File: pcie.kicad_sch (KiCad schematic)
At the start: 12 parts, among them J8 Conn_01x16_MountingPin

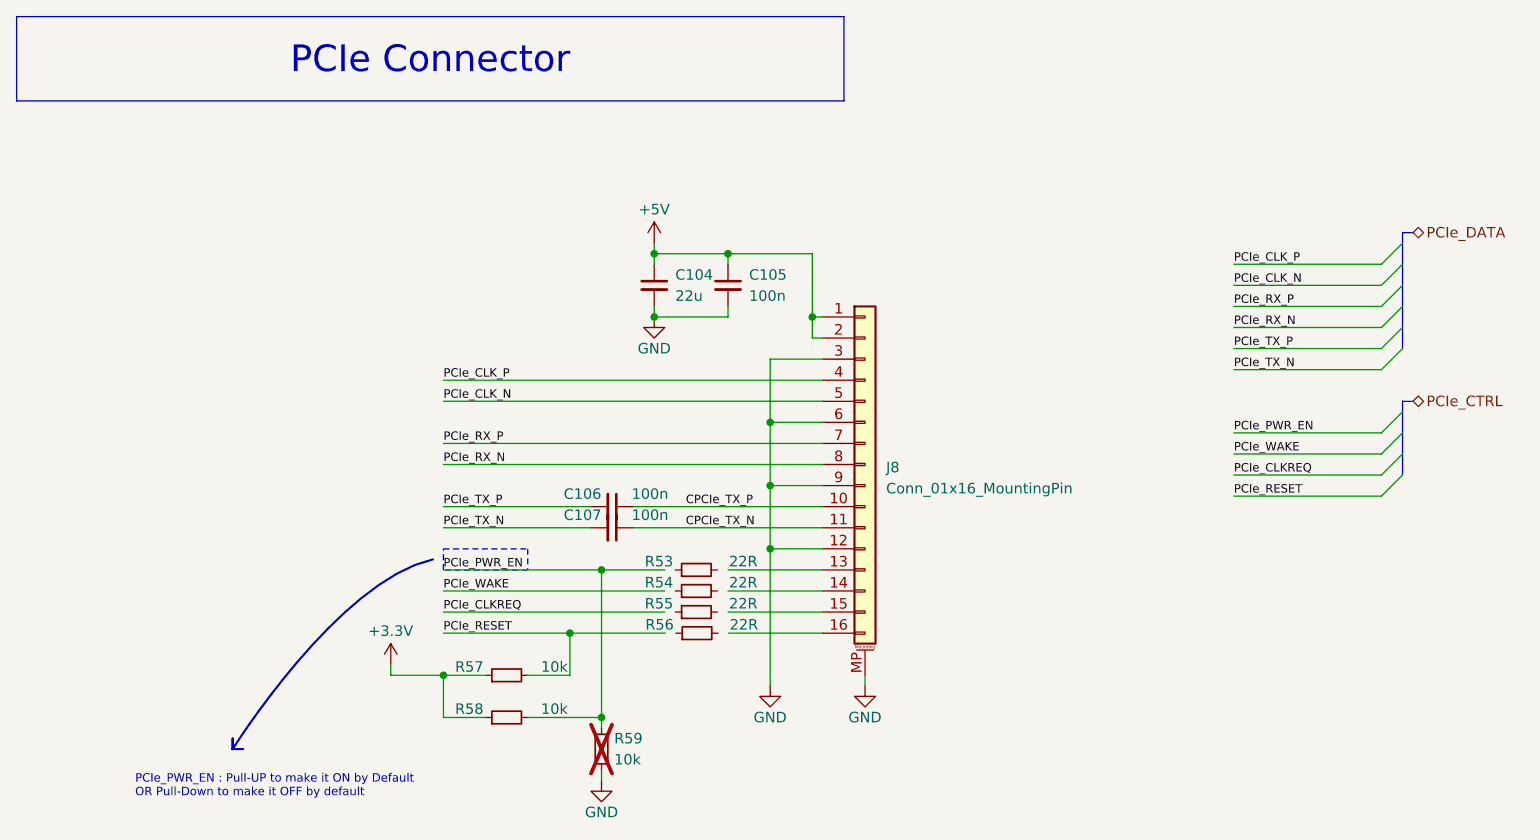
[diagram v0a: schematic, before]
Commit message: Add files via upload
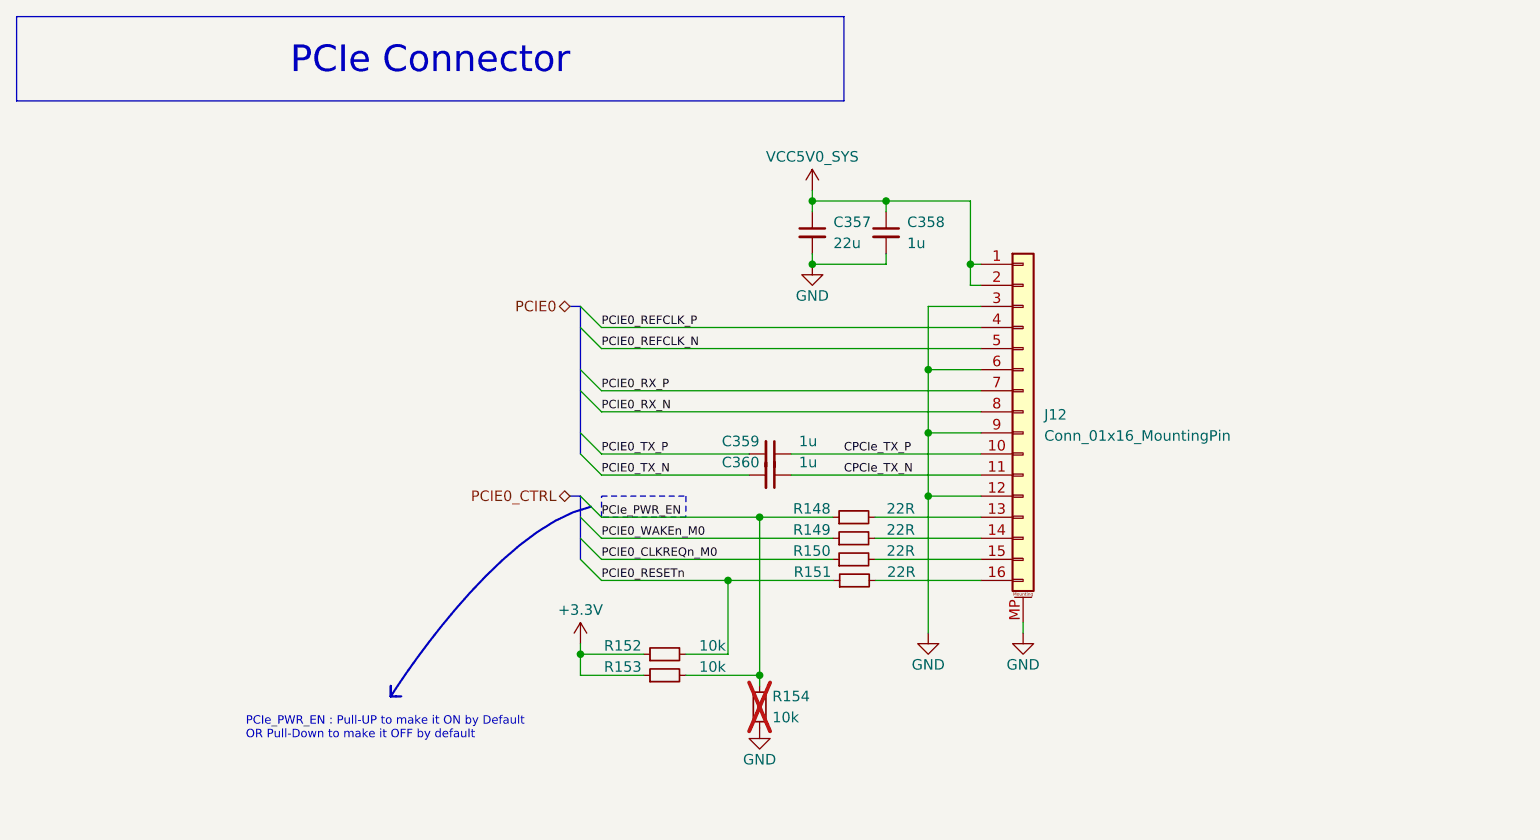
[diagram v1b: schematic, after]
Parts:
- C358: renamed from C105; value 100n -> 1u
- C359: renamed from C106; value 100n -> 1u
- C360: renamed from C107; value 100n -> 1u
- renumbered C104 to C357, J8 to J12, R53 to R148, R54 to R149, R55 to R150, R56 to R151, R57 to R152, R58 to R153, R59 to R154
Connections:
- net PCIe_RESET is gone; now on net PCIE0_RESETn: R152.2
- net PCIe_PWR_EN: now also R148.1
- net PCIE0_WAKEn_M0: now reaches R149.1
- net at R149.2: now also J12.14 (Pin_14)
- net PCIE0_CLKREQn_M0: now reaches R150.1
- net at R150.2: now also J12.15 (Pin_15)
- net PCIE0_RESETn: now reaches R151.1
- net at R151.2: now also J12.16 (Pin_16)
- net at R148.2: now also J12.13 (Pin_13)
- net +5V renamed VCC5V0_SYS
- net PCIe_CLK_N renamed PCIE0_REFCLK_N
- net PCIe_CLK_P renamed PCIE0_REFCLK_P
- net PCIe_RX_N renamed PCIE0_RX_N
- net PCIe_RX_P renamed PCIE0_RX_P
- net PCIe_TX_N renamed PCIE0_TX_N
- net PCIe_TX_P renamed PCIE0_TX_P
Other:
- moved on the sheet: C357, C358, C359, C360, J12, R148, R149, R150, R151, R152, R153, R154
